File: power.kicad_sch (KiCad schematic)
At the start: 7 parts, among them J13 Power Jumper, J8 ATX-24

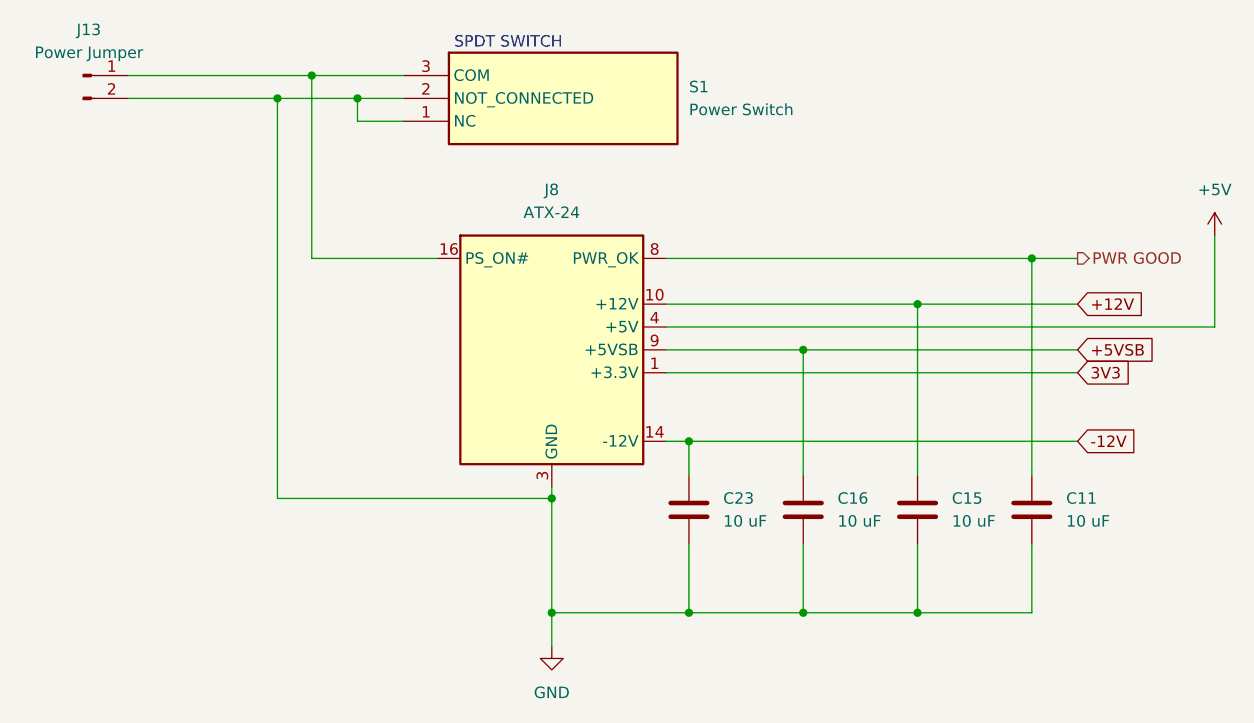
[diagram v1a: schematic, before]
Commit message: final commit before spinning
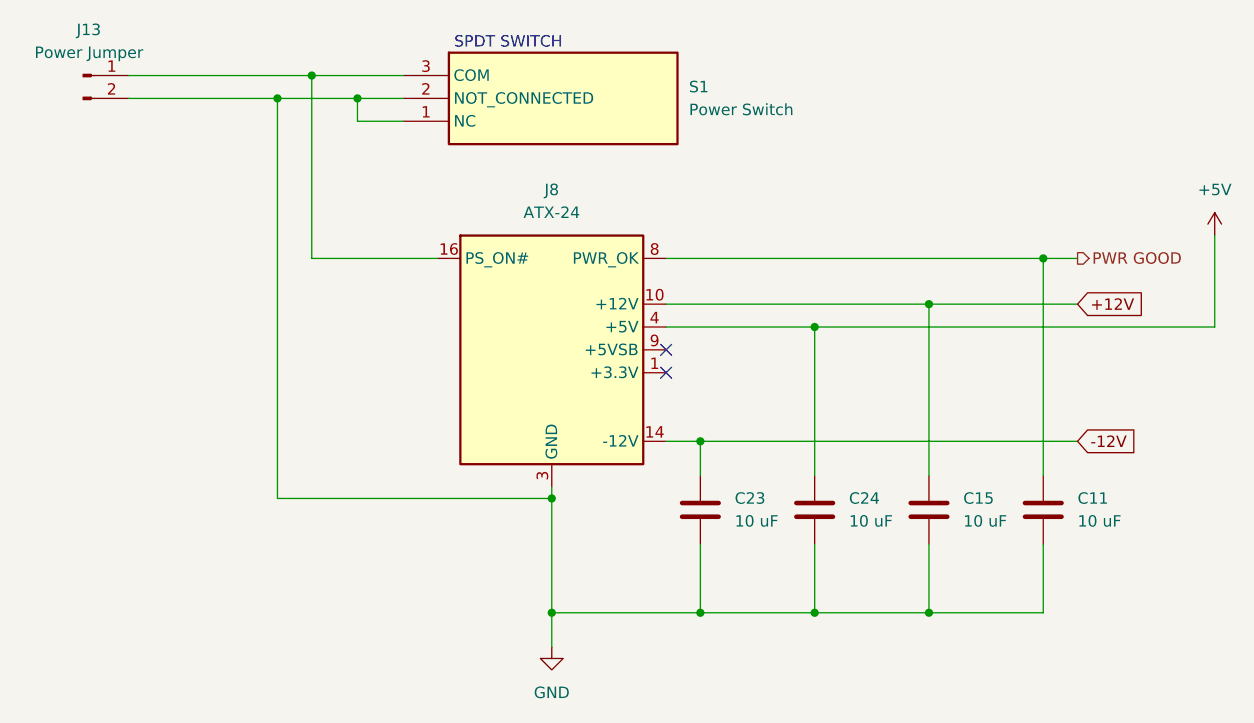
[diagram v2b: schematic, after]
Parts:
- removed C16: 10 uF, Capacitor_SMD:C_1210_3225Metric_Pad1.33x2.70mm_HandSolder, symbol Device:C
- added C24: 10 uF, Capacitor_SMD:C_1210_3225Metric_Pad1.33x2.70mm_HandSolder, symbol Device:C
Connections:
- net +5V: now also C24.1
- net GND: now also C24.2
- net +5VSB: no longer names the net of J8.9 (+5VSB)
- net 3V3: no longer names the net of J8.1 (+3.3V), J8.12 (+3.3V), J8.13 (+3.3V), J8.2 (+3.3V)
- no-connect marks 0 -> 2
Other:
- moved on the sheet: C11, C15, C23
